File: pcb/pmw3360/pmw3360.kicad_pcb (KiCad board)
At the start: 2 copper layers, 22 x 30 mm, 20 parts, among them J1 Connector, J2 PinOut, U1 PMW3360DM-T2QU, U2 TCR2EF19,LM(CT, U3 SN74LVC1T45QDCKRQ1, U4 TXB0104RUT

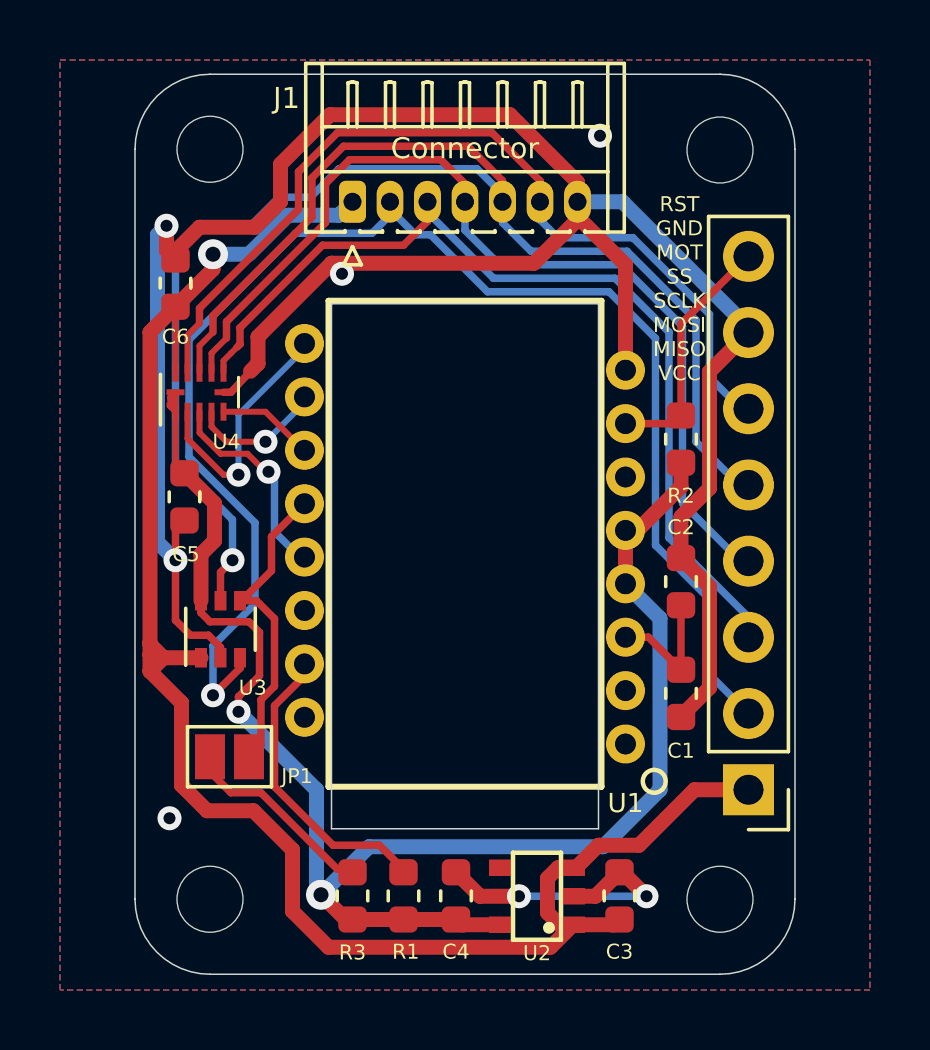
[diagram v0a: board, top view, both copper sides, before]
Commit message: change route
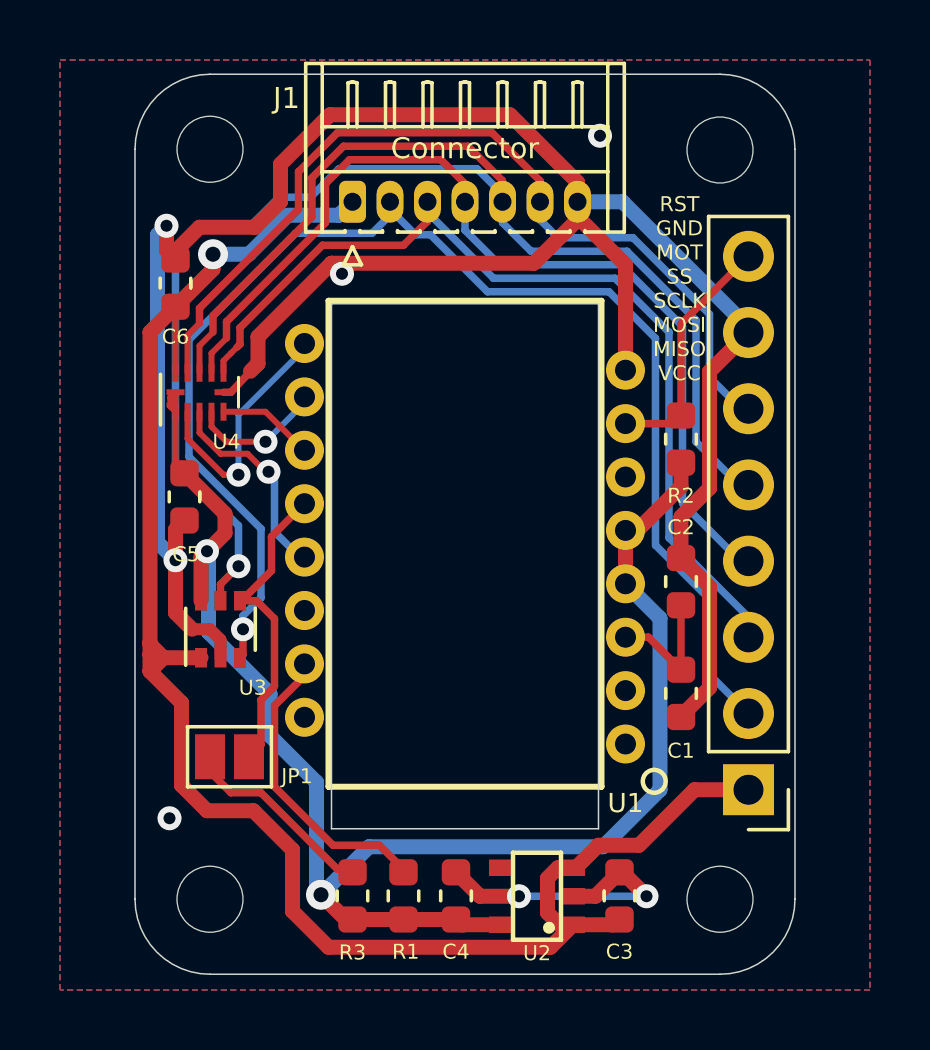
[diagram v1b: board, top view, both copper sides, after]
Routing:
- net /MISO-H: track 48.5 -> 45.4 mm
- net VDD: track 53.1 -> 53.6 mm
